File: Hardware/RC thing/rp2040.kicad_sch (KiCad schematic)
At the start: 27 parts, among them P1 USB_C_Plug_USB2.0, SW1 TL3342F160QG_TR, U2 RP2040, U3 W25Q128JVS, Y1 12Mhz

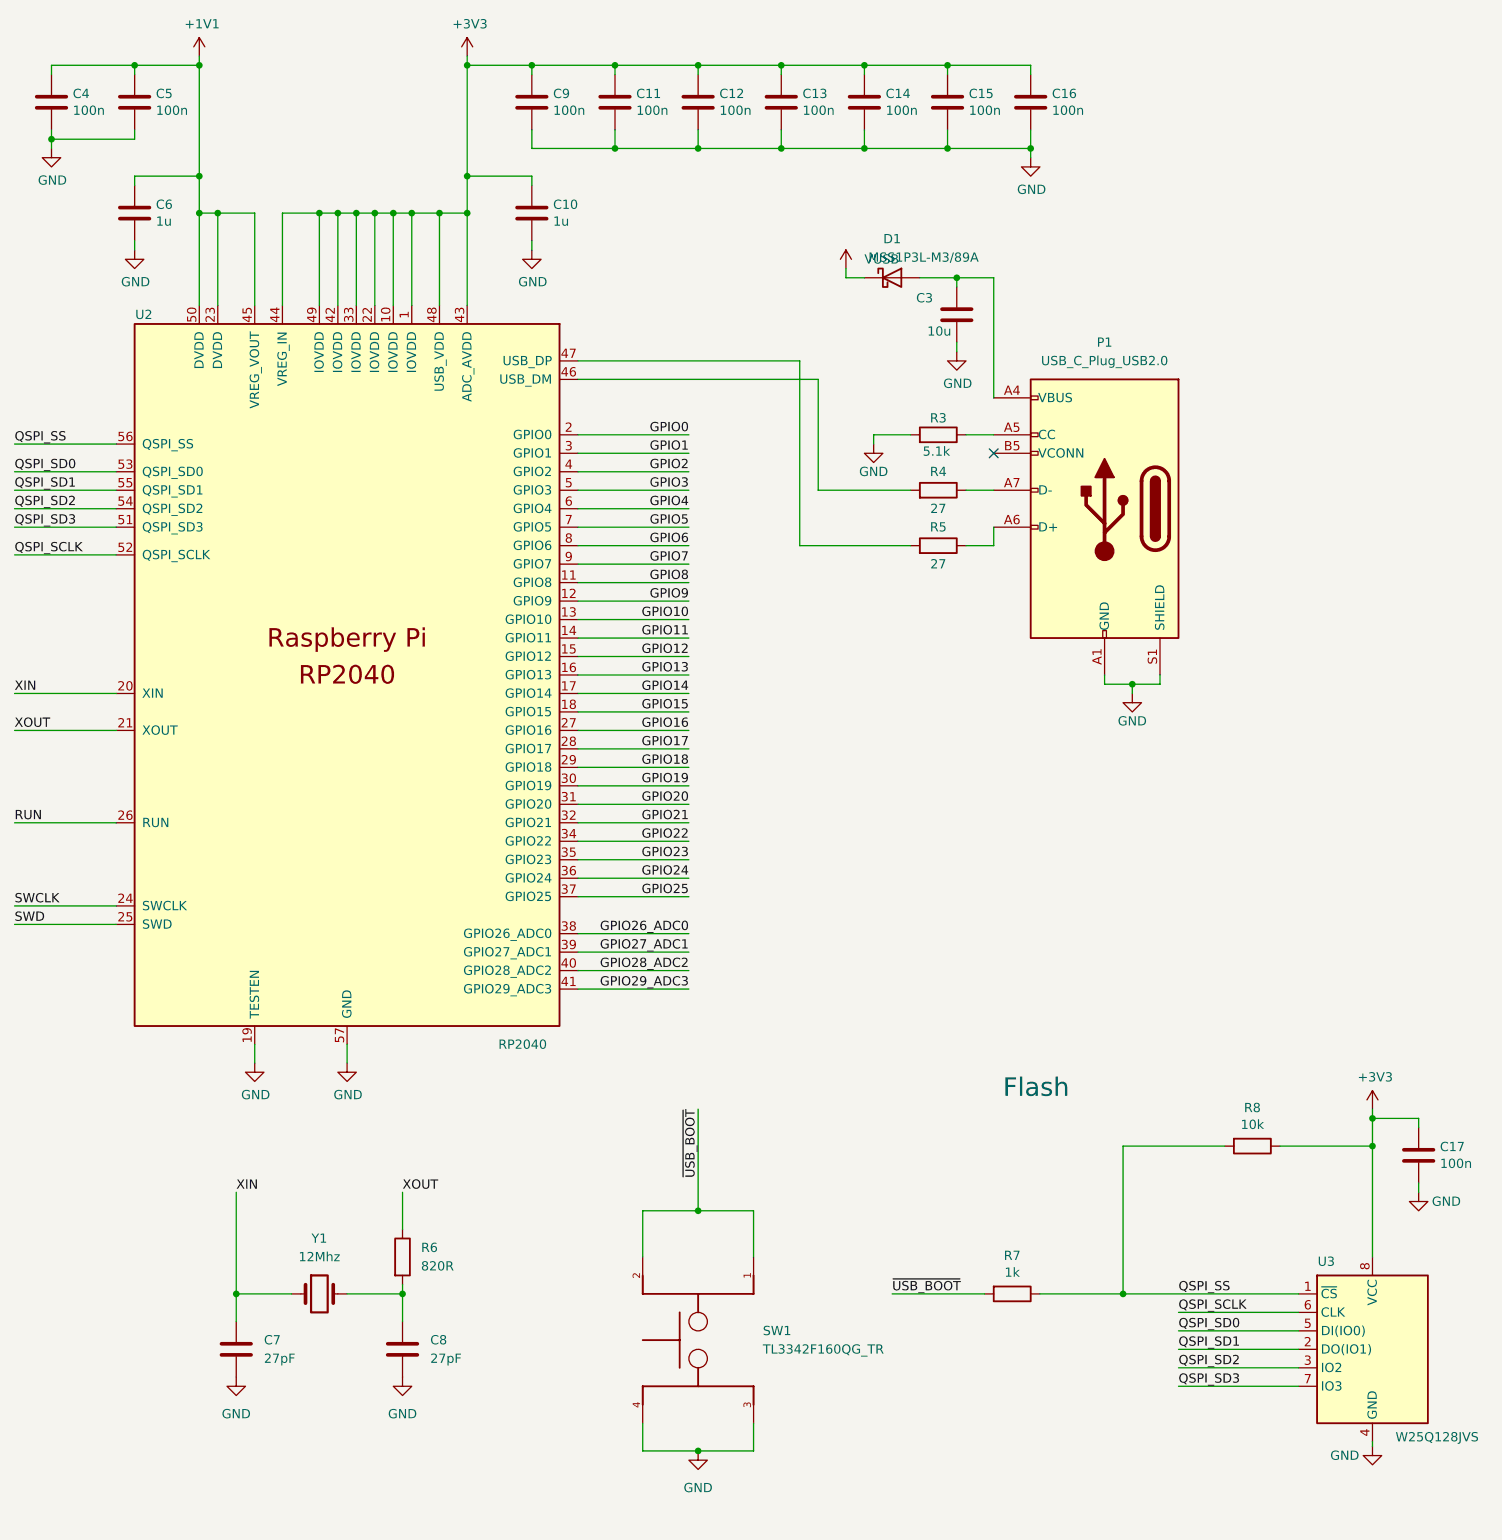
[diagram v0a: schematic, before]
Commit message: RC thing PCB 95% trustworthy (six seven)
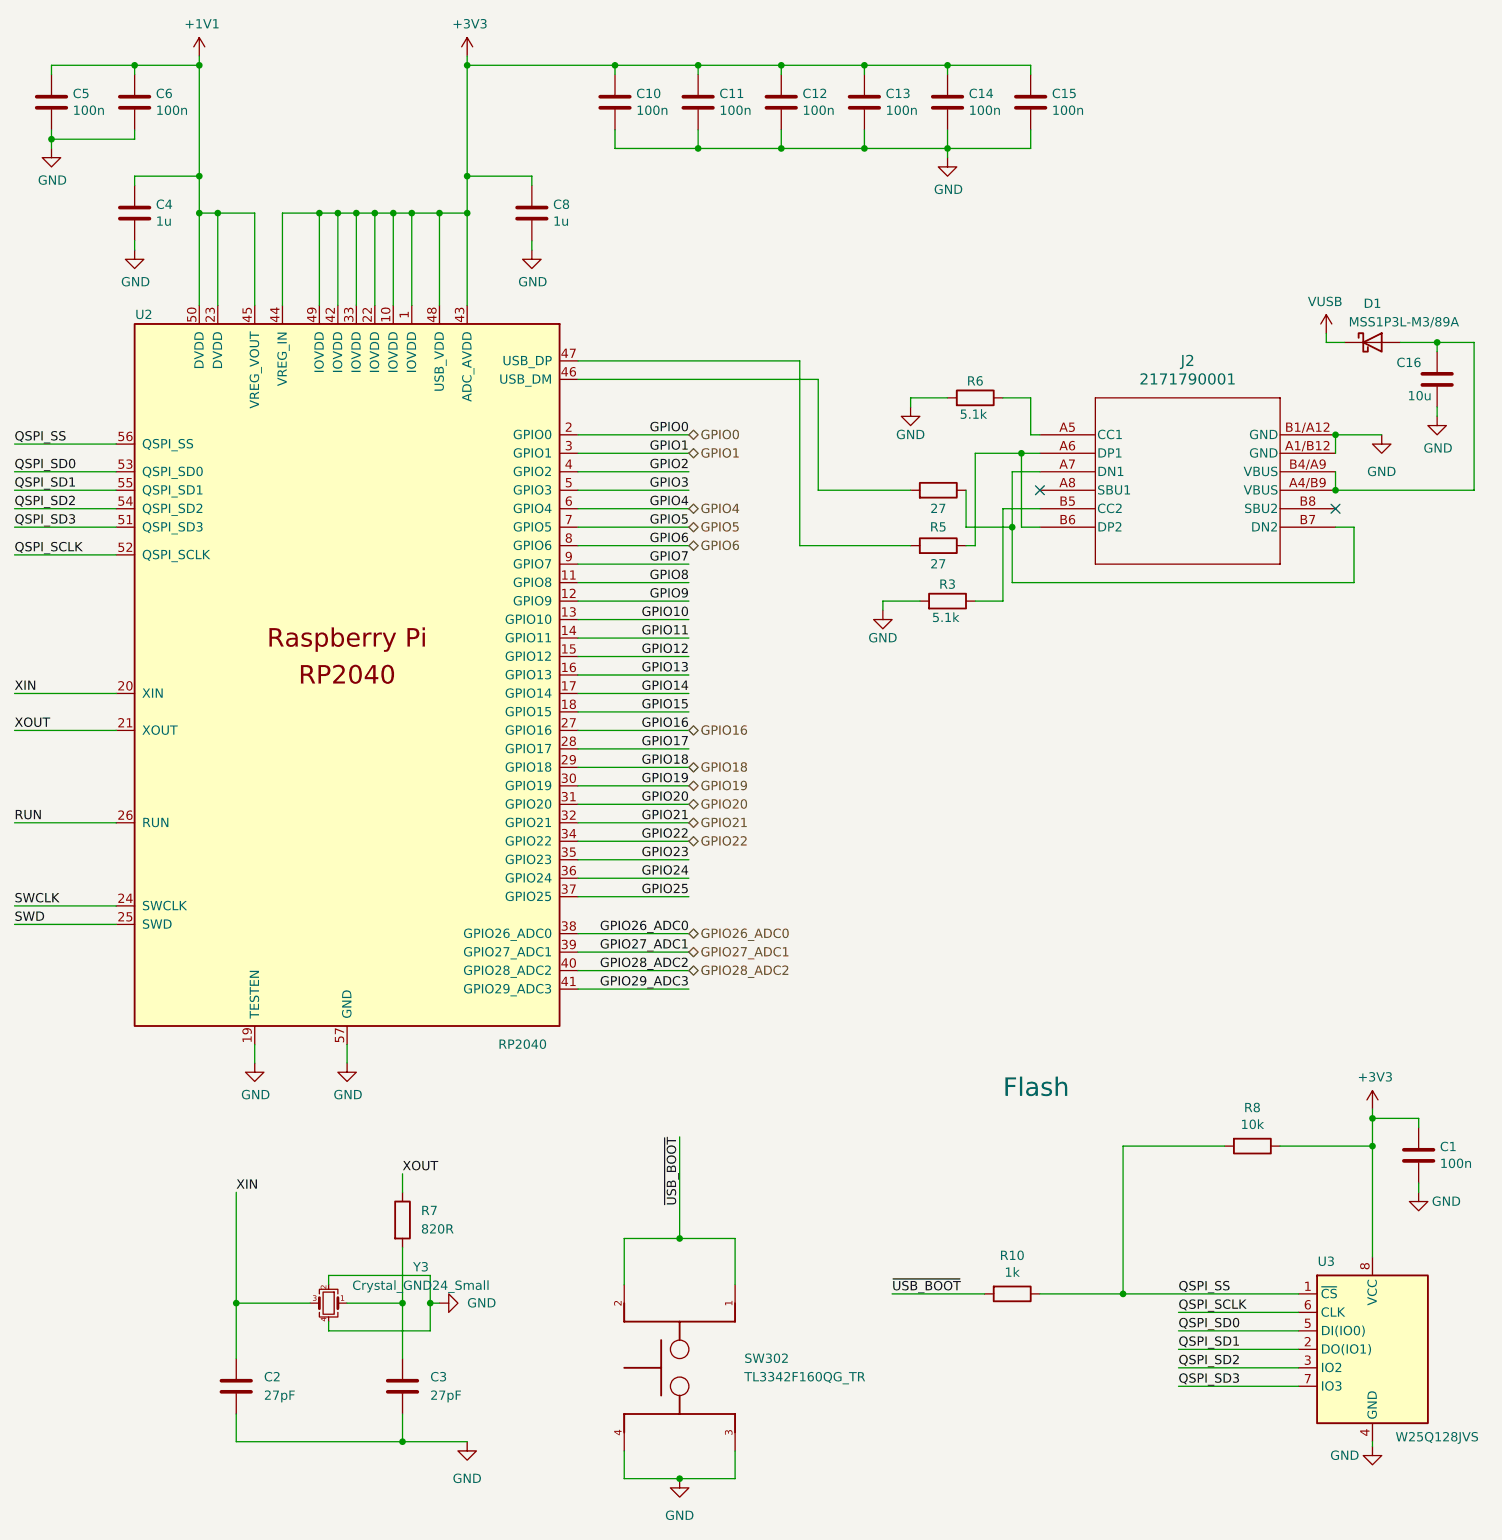
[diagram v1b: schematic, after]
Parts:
- removed C11: 100n, Capacitor_SMD:C_0603_1608Metric_Pad1.08x0.95mm_HandSolder, symbol Device:C
- removed P1: USB_C_Plug_USB2.0, Connector_USB:USB_C_Receptacle_Molex_105450-0101, symbol Connector:USB_C_Plug_USB2.0
- removed Y1: 12Mhz, Crystal:Crystal_SMD_Abracon_ABM8G-4Pin_3.2x2.5mm, symbol Device:Crystal
- added J2: 2171790001, rctg:2171790001_MOL, symbol MainPCB_Sym_lib:2171790001
- added R6: 5.1k, Resistor_SMD:R_0603_1608Metric_Pad0.98x0.95mm_HandSolder, symbol Device:R
- added Y3: Crystal_GND24_Small, Crystal:Crystal_SMD_Abracon_ABM8G-4Pin_3.2x2.5mm, symbol Device:Crystal_GND24_Small
- R10: renamed from R7; footprint Resistor_SMD:R_0402_1005Metric -> Resistor_SMD:R_0603_1608Metric_Pad0.98x0.95mm_HandSolder
- R7: renamed from R6; footprint (none) -> Resistor_SMD:R_0603_1608Metric_Pad0.98x0.95mm_HandSolder
- R8: footprint Resistor_SMD:R_0402_1005Metric -> Resistor_SMD:R_0603_1608Metric_Pad0.98x0.95mm_HandSolder
- SW302: renamed from SW1; footprint TL3342F160QG_TR:SW_TL3342F160QG_TR -> Main_PCB:SW_TL3342F160QG_TR
- U2: footprint RP2040_minimal:RP2040-QFN-56 -> Package_DFN_QFN:QFN-56-1EP_7x7mm_P0.4mm_EP3.2x3.2mm
- U3: footprint Package_SO:SOIC-8_5.23x5.23mm_P1.27mm -> Package_SO:SOIC-8_5.3x5.3mm_P1.27mm
- renumbered C17 to C1, C12 to C10, C13 to C11, C14 to C12, C15 to C13, C16 to C14, C9 to C15, C3 to C16, C7 to C2, C8 to C3, C6 to C4, C4 to C5, C5 to C6, C10 to C8
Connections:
- net GND: now also J2.A1/B12 (GND), J2.B1/A12 (GND), R6.2, Y3.2, Y3.4
- net XIN: now also Y3.3
- net at C3.1, R7.2: now also Y3.1
- net at C16.1, D1.2 (A): now also J2.A4/B9 (VBUS), J2.B4/A9 (VBUS)
- net at R4.1: now also J2.A7 (DN1), J2.B7 (DN2)
- net at R5.1: now also J2.A6 (DP1), J2.B6 (DP2)
- net at R3.1: now also J2.B5 (CC2)
- new net: J2.A5 (CC1), R6.1
- no-connect marks 1 -> 2
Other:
- moved on the sheet: C10, C11, C12, C13, C14, C15, C16, C2, C3, D1, R3, R7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
